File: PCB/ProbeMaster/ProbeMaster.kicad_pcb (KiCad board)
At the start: 2 copper layers, 63.5 x 101.6 mm, 215 parts, among them J1 Conn_01x08_Male, J10 Conn_01x08_Male, J11 Conn_01x08_Male, J12 Screw_Terminal_01x08, J2 Conn_01x08_Male, J3 Conn_01x08_Male, J4 Conn_01x08_Male, J5 Screw_Terminal_01x08, J6 Screw_Terminal_01x08, J7 Screw_Terminal_01x08, J8 Conn_01x08_Male, J9 Conn_01x08_Male, SW1 SW_DIP_x08

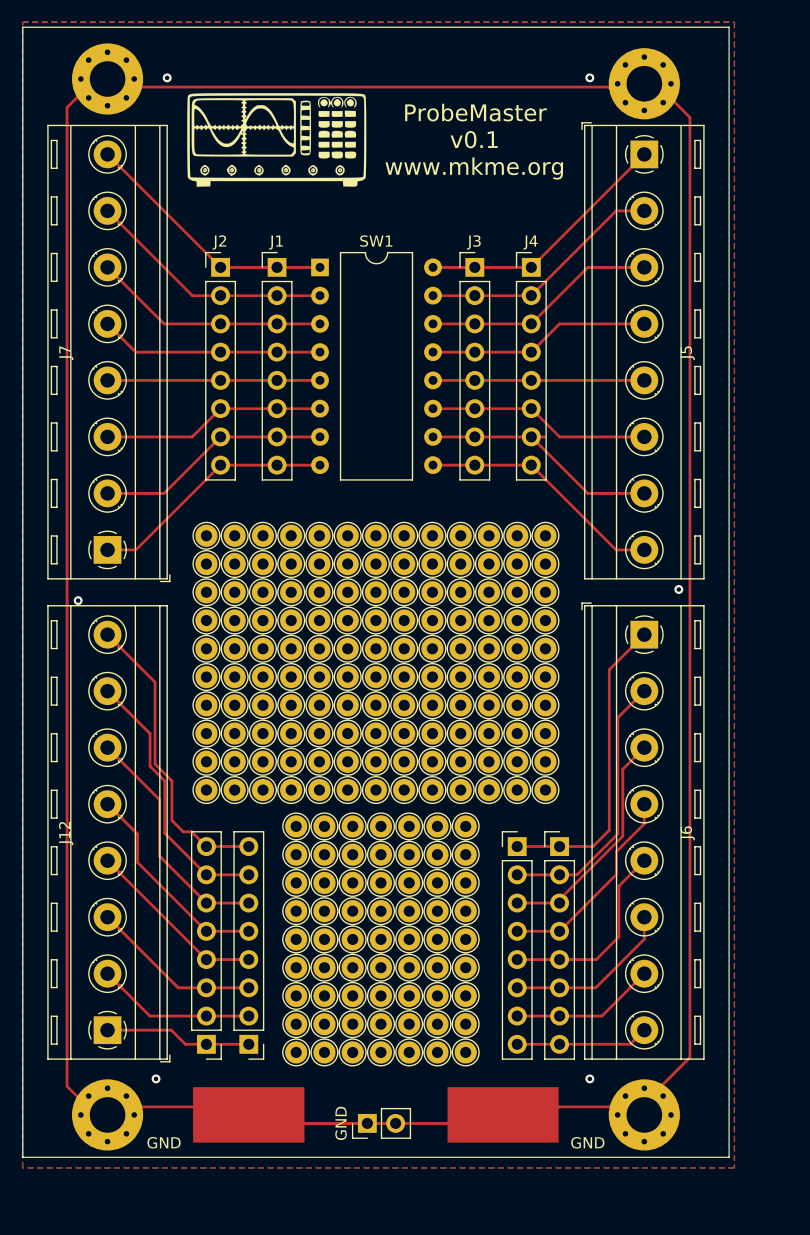
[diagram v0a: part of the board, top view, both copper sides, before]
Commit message: update edgecuts
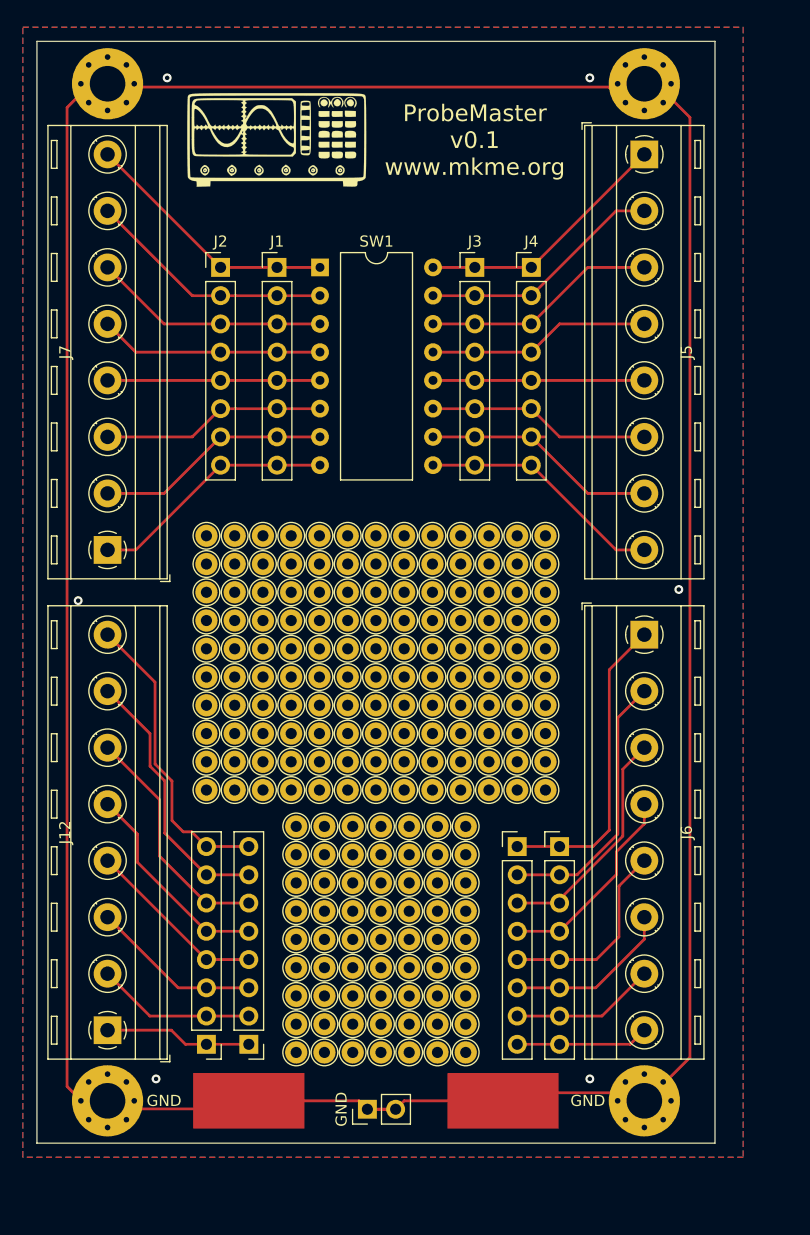
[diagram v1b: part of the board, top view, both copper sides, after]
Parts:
- moved GND 1.27 mm to (203.2, 141.0)
- moved GND 1.27 mm to (191.0, 141.7)
- moved REF** 1.27 mm to (180.3, 141.0)
- moved REF** 1.27 mm to (167.6, 141.0)
- moved REF** 1.27 mm to (215.9, 141.0)
- moved REF** 0.43 mm to (167.6, 49.5)
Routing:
- net GND: track 298.3 -> 301.8 mm
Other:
- board size 63.5 x 101.6 mm -> 61 x 99.1 mm
